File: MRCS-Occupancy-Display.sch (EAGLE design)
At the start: 8 parts, among them CON1 CONNECTOR-M12LOCK, CON2 CONNECTOR-M12LOCK, IC1 74ALS04N

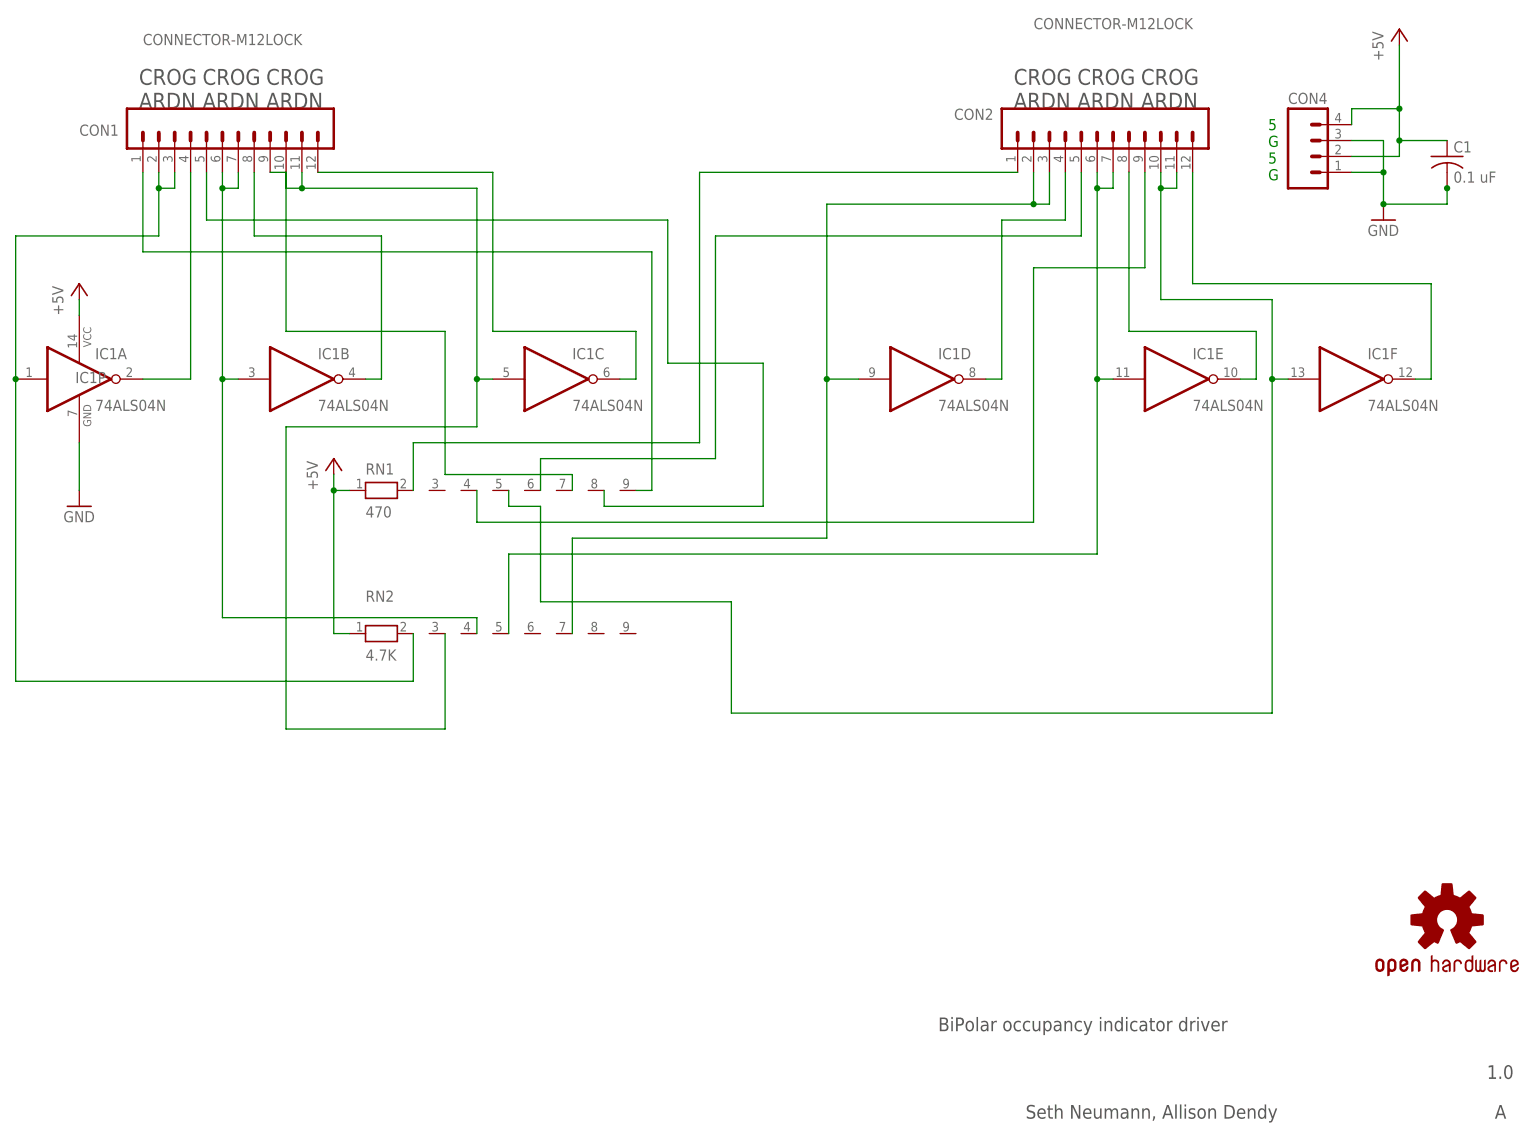
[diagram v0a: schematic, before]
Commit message: cleanup prior to putting product up on website
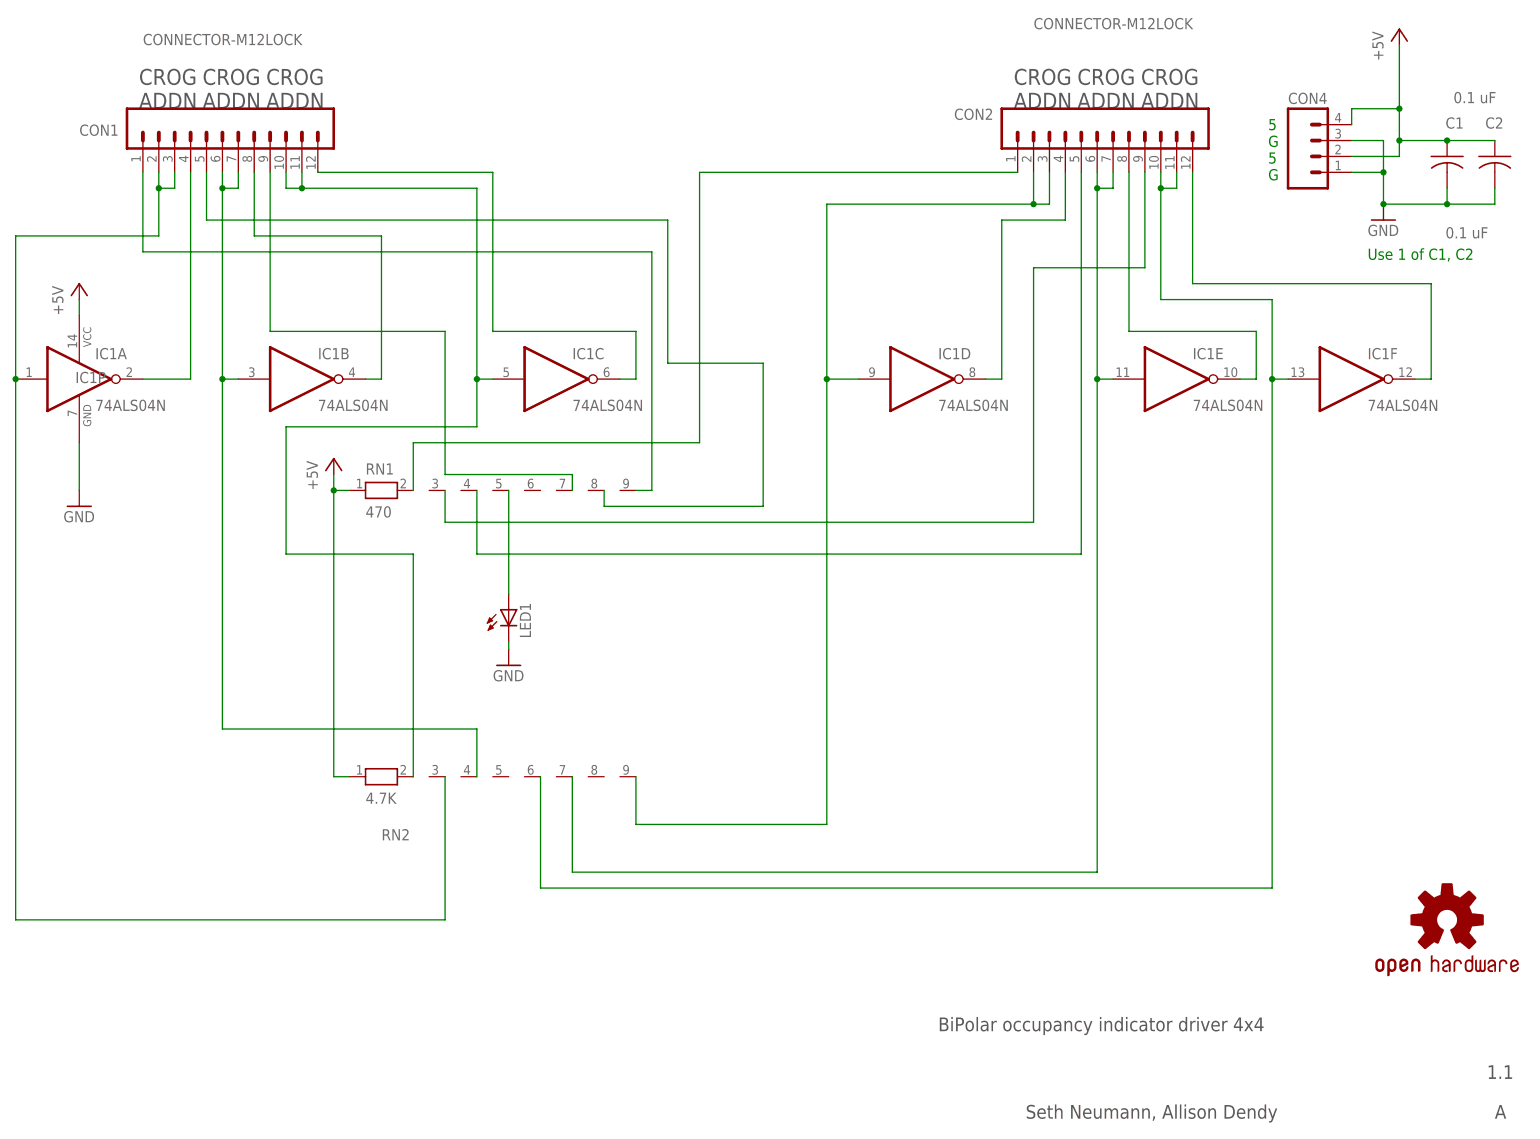
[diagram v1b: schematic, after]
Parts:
- added C2: 0.1 uF, SPCoast:CAPPTH1
- added LED1: (no value), SPCoast:LEDLED3MM
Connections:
- removed net N$1: CON1.2, CON1.3, IC1A.I, RN2.2
- new net N$16: CON1.2, CON1.3, IC1A.I, RN2.3
- new net N$17: LED1.A, RN1.5
- net GND: now also C2.2, LED1.C
- net N$15: now also RN1.4; no longer RN1.6
- net N$18: now also RN2.7; no longer RN2.5
- net N$19: now also RN1.3; no longer RN1.4
- net N$2: now also RN2.2; no longer RN2.3
- net N$20: now also RN2.6; no longer RN1.5
- net N$9: now also RN2.9; no longer RN2.7
- net VCC: now also C2.1
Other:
- note added: "1.1"
- note added: "BiPolar occupancy indicator driver 4x4"
- note added: "CROG ADDN"
- note added: "Use 1 of C1, C2"
- note removed: "1.0"
- note removed: "BiPolar occupancy indicator driver"
- note removed: "CROG ARDN"
- moved on the sheet: RN2
